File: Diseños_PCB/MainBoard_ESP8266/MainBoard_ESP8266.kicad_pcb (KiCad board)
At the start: 2 copper layers, 60 x 60 mm, 37 parts, among them J1 Input_BAT, J2 USB_B_Micro, J3 FTDI, Q1 2N7002, SW1 SW_SPDT, SW2 SW_Push, SW3 SW_Push, U2 AMS1117-3.3, U3 ESP-12F, U4 MT3608, U5 TP4056

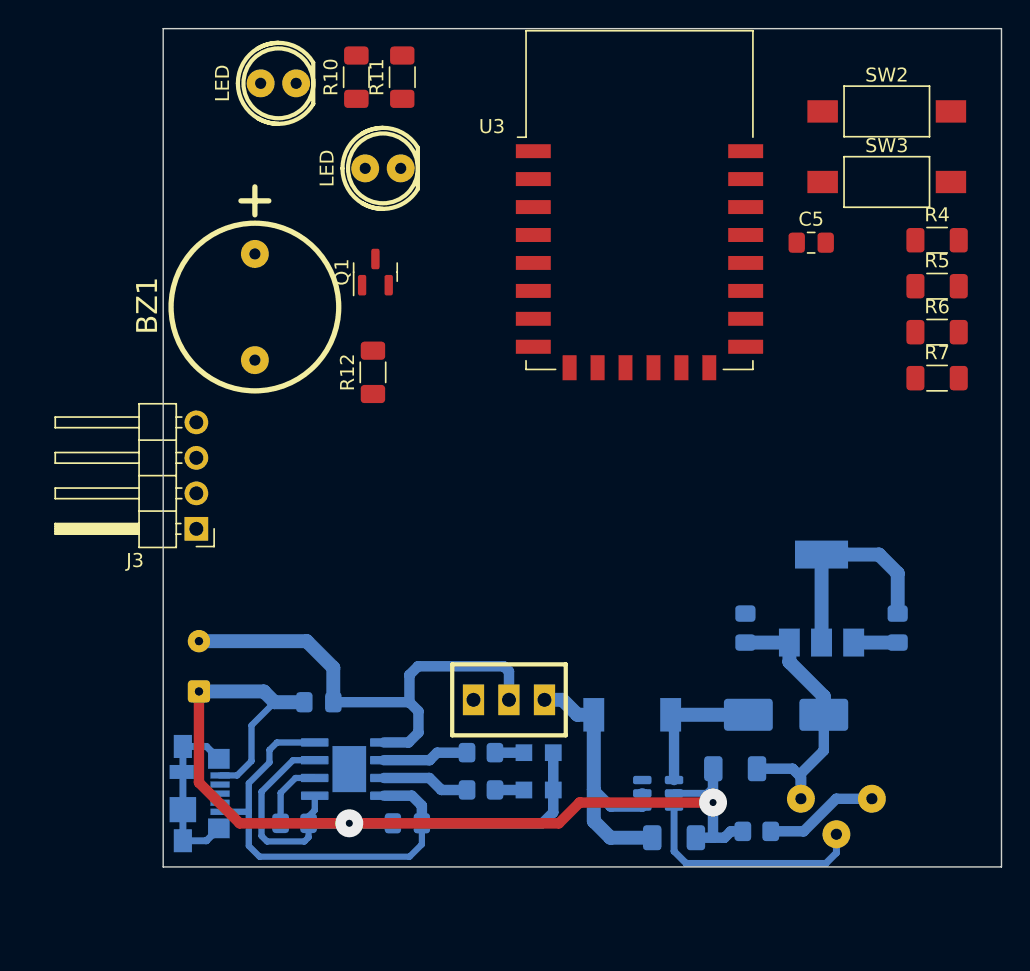
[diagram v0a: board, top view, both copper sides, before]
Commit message: Edicion archivos pcb
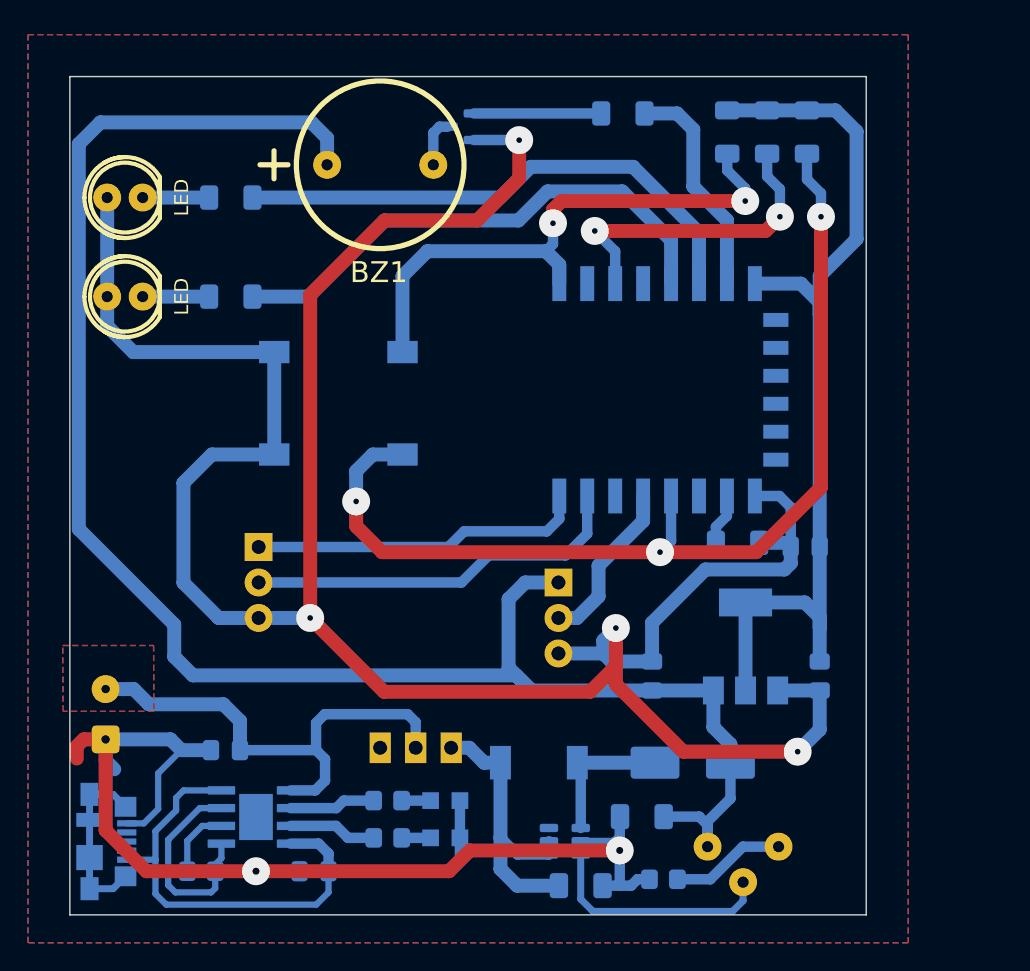
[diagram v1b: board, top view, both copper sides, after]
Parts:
- removed J3: FTDI, Connector_PinHeader_2.54mm:PinHeader_1x04_P2.54mm_Horizontal
- added J4: Sensor, Connector_PinHeader_2.54mm:PinHeader_1x03_P2.54mm_Horizontal, B.Cu at (155.3, 106.6)
- added J5: FTDI, Connector_PinHeader_2.54mm:PinHeader_1x03_P2.54mm_Horizontal, B.Cu at (133.8, 104.1)
- C5, Q1, R10, R11, R12, R4, R5, R6, R7, SW1, SW2, SW3, U3: moved to B.Cu
- moved SW3 43.8 mm to (139.5, 97.5), turned to 180 degrees
- moved SW2 42.9 mm to (139.5, 90.2)
- moved R12 25.8 mm to (159.9, 73.1), turned to 180 degrees
- moved C5 21.8 mm to (173.0, 104.1)
- moved D5 20.6 mm to (124.3, 86.2)
- moved R11 19.9 mm to (131.8, 86.2), turned to 180 degrees
- moved R5 18.6 mm to (167.4, 74.4), turned to -90 degrees
- moved R7 18.5 mm to (168.1, 103.8)
- moved R6 17.1 mm to (173.1, 74.4), turned to -90 degrees
- moved R4 14.4 mm to (170.2, 74.4), turned to -90 degrees
- moved U3 13.8 mm to (158.8, 92.8), turned to -90 degrees
- moved D4 13.7 mm to (124.3, 79.1)
- moved BZ1 13.6 mm to (142.5, 76.7), turned to 180 degrees
- moved R10 12.4 mm to (131.8, 79.1), turned to 180 degrees
- moved Q1 12.1 mm to (148.3, 74.0), turned to 180 degrees
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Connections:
- U3 pad 19: unconnected-(U3-GPIO4-Pad19) -> /PIR
- U3 pad 5: /BUZZER -> /LED_WIFI
- U3 pad 7: /LED_WIFI -> /BUZZER
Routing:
- net GND: track 97.3 -> 288.9 mm, vias 2 -> 6
- net +5V: track 21.0 -> 128.5 mm
- net Net-(U3-GPIO0): track 0.00 -> 72.4 mm, vias 0 -> 3
- net +3.3V: track 15.2 -> 67.8 mm
- net Net-(U3-~{RST}): track 0.00 -> 40.3 mm, vias 0 -> 2
- net /LED_STATUS: track 0.00 -> 38.5 mm
- net /LED_WIFI: track 0.00 -> 37.6 mm
- net /Rx: track 0.00 -> 27.7 mm
- net /Tx: track 0.00 -> 24.0 mm
- net Net-(U3-EN): track 0.00 -> 22.9 mm, vias 0 -> 2
- net /BUZZER: track 0.00 -> 16.0 mm
- net /PIR: track 0.00 -> 12.0 mm
- net Net-(Q1-G): track 0.00 -> 9.11 mm
- net Net-(D5-A): track 0.00 -> 4.76 mm
- net Net-(D4-A): track 0.00 -> 4.76 mm
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- added copper zone on B.Cu, net /VB
- added copper zone on F.Cu, net /VB
- added copper zone on B.Cu, net GND
- added copper zone on F.Cu, net GND
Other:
- board size 60 x 60 mm -> 57 x 60 mm
